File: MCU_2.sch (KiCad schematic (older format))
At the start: 18 parts, among them U2 STM32F051K6Ux

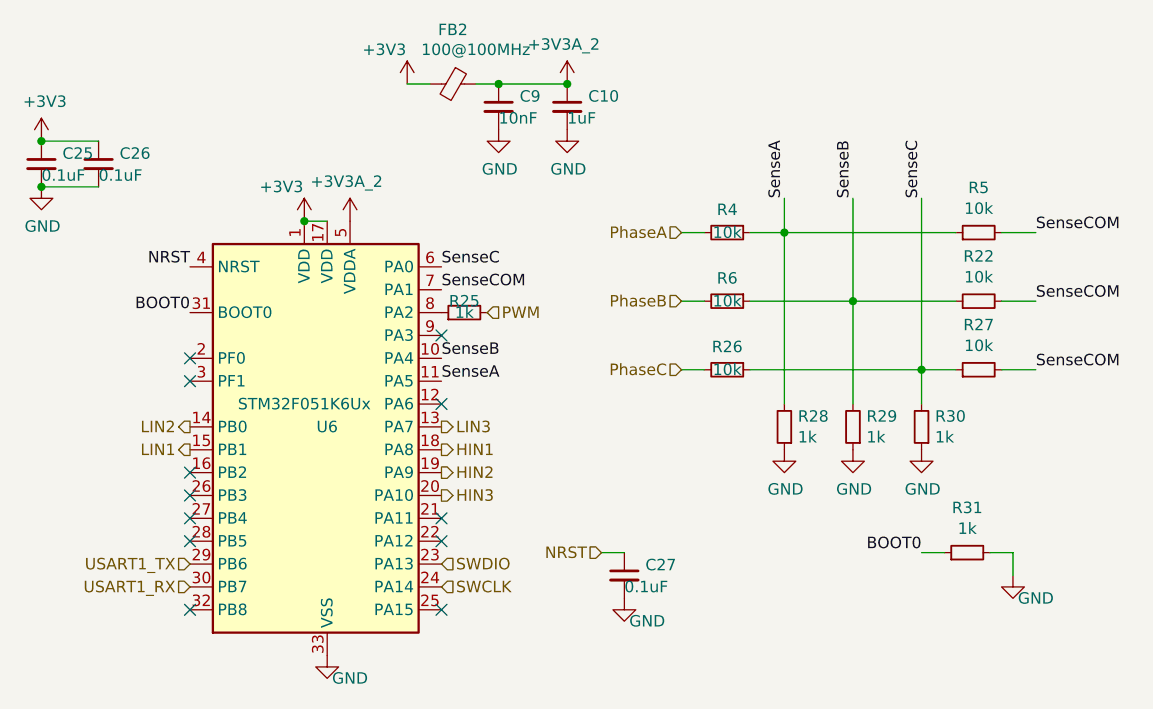
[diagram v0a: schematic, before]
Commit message: Added stuff
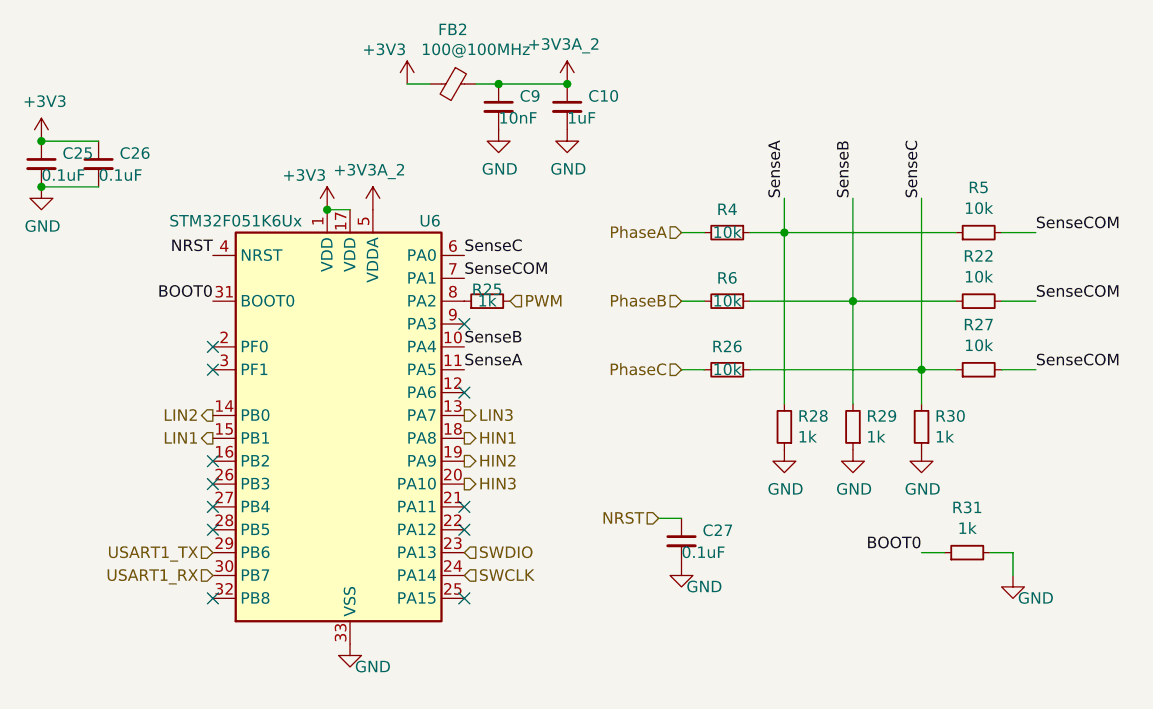
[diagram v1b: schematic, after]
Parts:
- removed R24: 1k, Resistor_SMD:R_0402_1005Metric, symbol Device:R_Small
- removed U2: STM32F051K6Ux, Package_DFN_QFN:QFN-32-1EP_5x5mm_P0.5mm_EP3.45x3.45mm, symbol MCU_ST_STM32F0:STM32F051K6Ux
- added R25: 1k, Resistor_SMD:R_0402_1005Metric, symbol Device:R_Small
- added U6: STM32F051K6Ux, Package_DFN_QFN:QFN-32-1EP_5x5mm_P0.5mm_EP3.45x3.45mm, symbol MCU_ST_STM32F0:STM32F051K6Ux
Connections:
- net +3.3VA_2: now also U6.5 (VDDA)
- net +3V3: now also U6.1 (VDD), U6.17 (VDD)
- net BOOT0: now also U6.31 (BOOT0)
- net GND: now also U6.33 (VSS)
- net HIN1: now also U6.18 (PA8)
- net HIN2: now also U6.19 (PA9)
- net HIN3: now also U6.20 (PA10)
- net LIN1: now also U6.15 (PB1)
- net LIN2: now also U6.14 (PB0)
- net LIN3: now also U6.13 (PA7)
- net NRST: now also U6.4 (NRST)
- net PWM: now also R25.2
- net SWCLK: now also U6.24 (PA14)
- net SWDIO: now also U6.23 (PA13)
- net SenseA: now also U6.11 (PA5)
- net SenseB: now also U6.10 (PA4)
- net SenseC: now also U6.6 (PA0)
- net SenseCOM: now also U6.7 (PA1)
- net USART1_RX: now also U6.30 (PB7)
- net USART1_TX: now also U6.29 (PB6)
- new net: R25.1, U6.8 (PA2)
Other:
- moved on the sheet: C27
